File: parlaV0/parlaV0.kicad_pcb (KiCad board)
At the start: 2 copper layers, 52.3 x 52.3 mm, 13 parts, among them U1 LM386

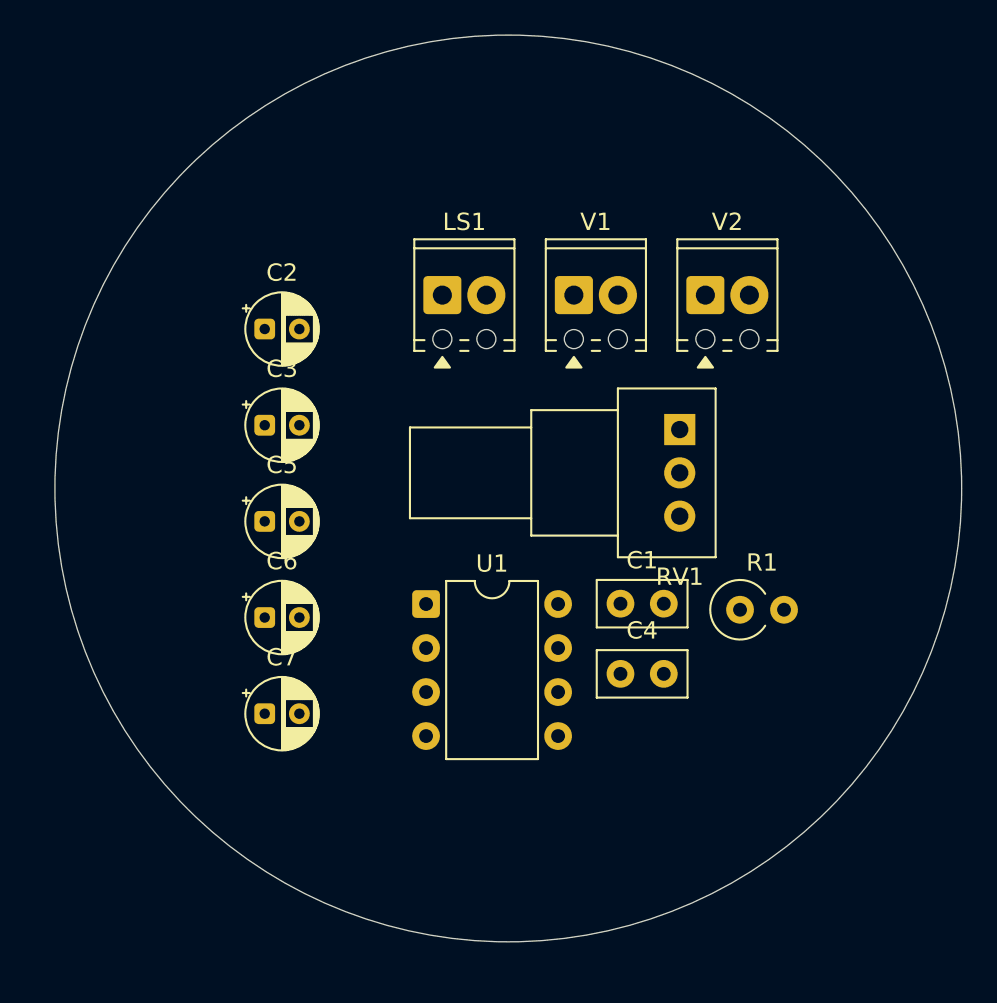
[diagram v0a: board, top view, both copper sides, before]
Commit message: agregar logo
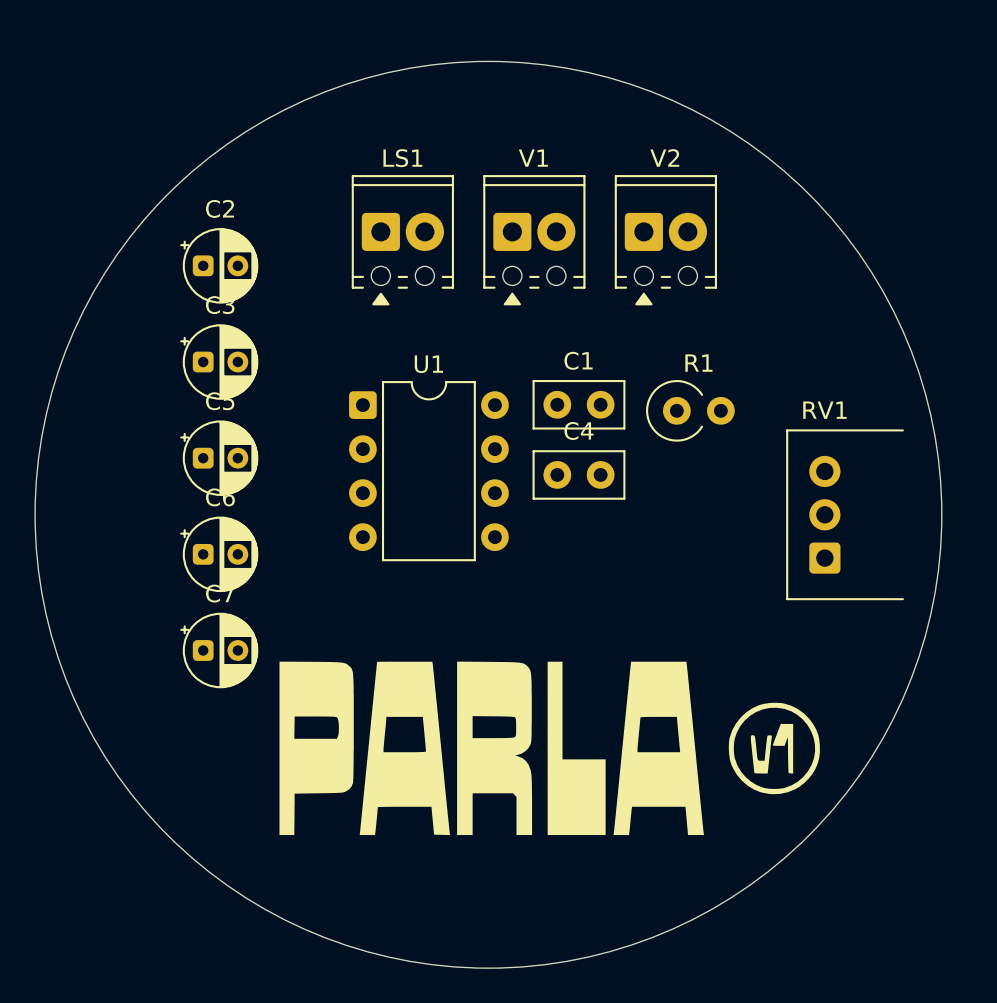
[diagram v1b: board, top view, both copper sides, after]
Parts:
- added  : LOGO, graficas:parla_logo, F.Cu at (120.0, 99.0)
- RV1: footprint Potentiometer_THT:Potentiometer_Alps_RK09Y11_Single_Horizontal -> Potentiometer_THT:Potentiometer_Alps_RK097_Single_Horizontal
- moved R1 12.0 mm to (127.3, 79.5)
- moved U1 12.0 mm to (109.2, 79.2)
- moved C1 12.0 mm to (120.4, 79.2)
- moved C4 12.0 mm to (120.4, 83.2)
- moved RV1 11.2 mm to (135.9, 88.0), turned to 180 degrees
- moved V1 5.09 mm to (117.8, 69.2)
- moved V2 5.09 mm to (125.4, 69.2)
- moved C5 5.09 mm to (100.0, 82.3)
- moved C6 5.09 mm to (100.0, 87.8)
- moved LS1 5.09 mm to (110.2, 69.2)
- moved C2 5.09 mm to (100.0, 71.2)
- moved C3 5.09 mm to (100.0, 76.7)
- moved C7 5.09 mm to (100.0, 93.4)
